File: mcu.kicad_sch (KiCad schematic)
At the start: 1 part, among them U1 PIC32CK1025GC01100-I/4SB

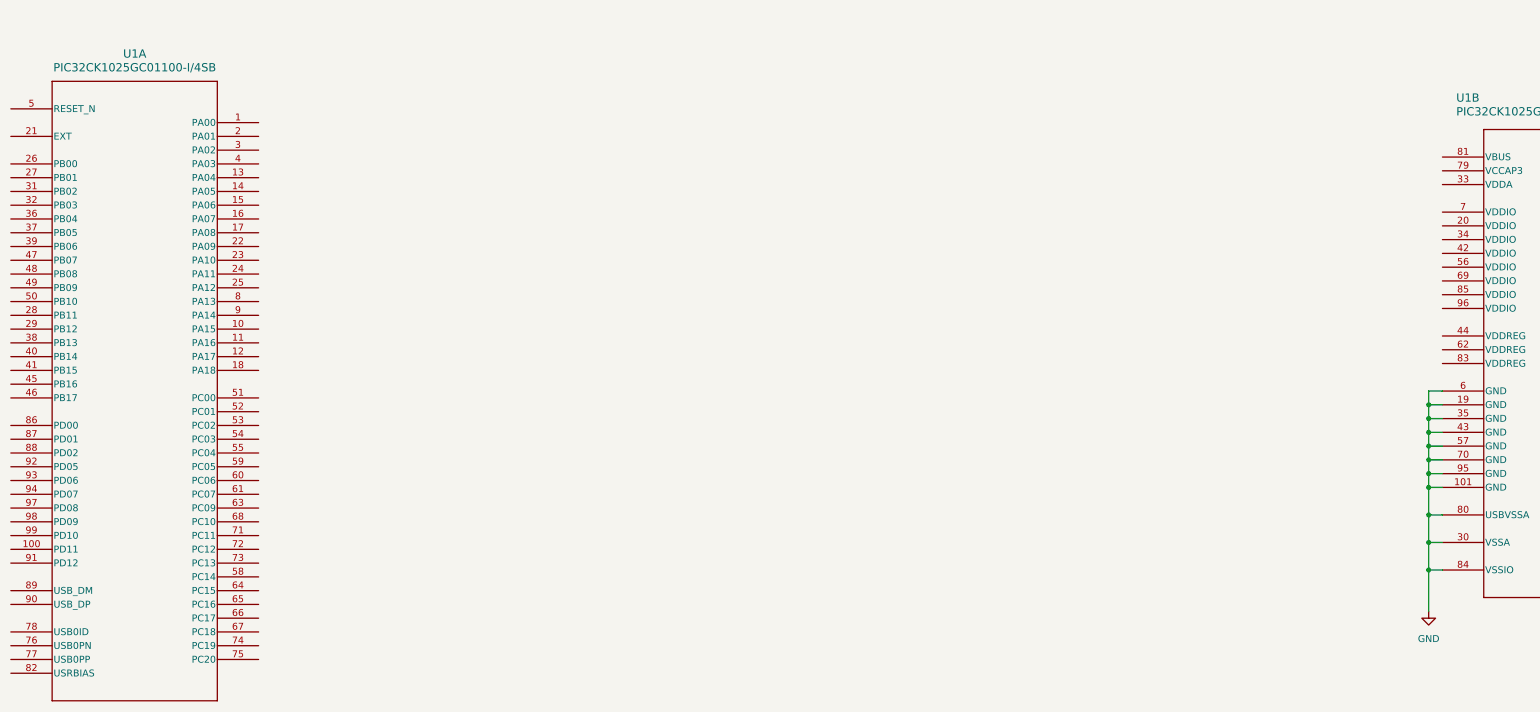
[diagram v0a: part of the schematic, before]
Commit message: did stuff
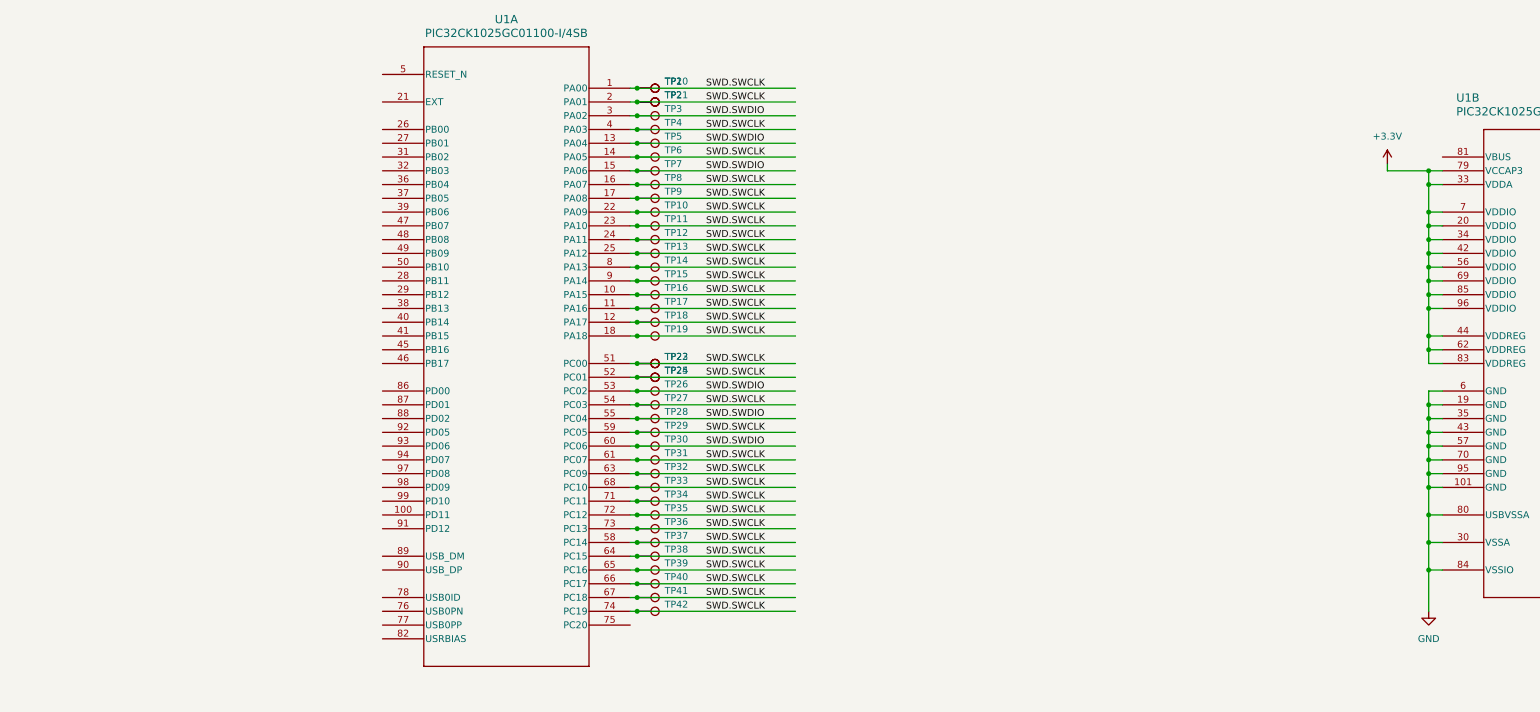
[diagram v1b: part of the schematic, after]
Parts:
- added TP1, TP10, TP11, TP12, TP13, TP14, TP15, TP16, TP17, TP18, TP19, TP2, TP20, TP21, TP22, TP23, TP24, TP25, TP26, TP27, TP28, TP29, TP3, TP30, TP31, TP32, TP33, TP34, TP35, TP36, TP37, TP38, TP39, TP4, TP40, TP41, TP42, TP5, TP6, TP7, TP8, TP9: TestPoint, symbol Connector:TestPoint
- U1: footprint TQFP100_4SB_6p3EP_MCH -> PIC32CK1025GC01100-I-4SB:TQFP100_4SB_6p3EP_MCH
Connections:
- net +3.3V: now reaches U1.20 (VDDIO)
- net +3.3V: now also U1.33 (VDDA), U1.34 (VDDIO), U1.42 (VDDIO), U1.44 (VDDREG), U1.56 (VDDIO), U1.62 (VDDREG), U1.69 (VDDIO), U1.7 (VDDIO), U1.79 (VCCAP3), U1.83 (VDDREG), U1.85 (VDDIO), U1.96 (VDDIO)
- net SWD.SWCLK: now reaches U1.1 (PA00)
- net SWD.SWCLK: now also U1.10 (PA15), U1.11 (PA16), U1.12 (PA17), U1.14 (PA05), U1.16 (PA07), U1.17 (PA08), U1.18 (PA18), U1.2 (PA01), U1.22 (PA09), U1.23 (PA10), U1.24 (PA11), U1.25 (PA12), U1.4 (PA03), U1.51 (PC00), U1.52 (PC01), U1.54 (PC03), U1.58 (PC14), U1.59 (PC05), U1.61 (PC07), U1.63 (PC09), U1.64 (PC15), U1.65 (PC16), U1.66 (PC17), U1.67 (PC18), U1.68 (PC10), U1.71 (PC11), U1.72 (PC12), U1.73 (PC13), U1.74 (PC19), U1.8 (PA13), U1.9 (PA14), TP1.1, TP10.1, TP11.1, TP12.1, TP13.1, TP14.1, TP15.1, TP16.1, TP17.1, TP18.1, TP19.1, TP2.1, TP20.1, TP21.1, TP22.1, TP23.1, TP24.1, TP25.1, TP27.1, TP29.1, TP31.1, TP32.1, TP33.1, TP34.1, TP35.1, TP36.1, TP37.1, TP38.1, TP39.1, TP4.1, TP40.1, TP41.1, TP42.1, TP6.1, TP8.1, TP9.1
- net SWD.SWDIO: now reaches U1.13 (PA04)
- net SWD.SWDIO: now also U1.15 (PA06), U1.3 (PA02), U1.53 (PC02), U1.55 (PC04), U1.60 (PC06), TP26.1, TP28.1, TP3.1, TP30.1, TP5.1, TP7.1
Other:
- moved on the sheet: U1A

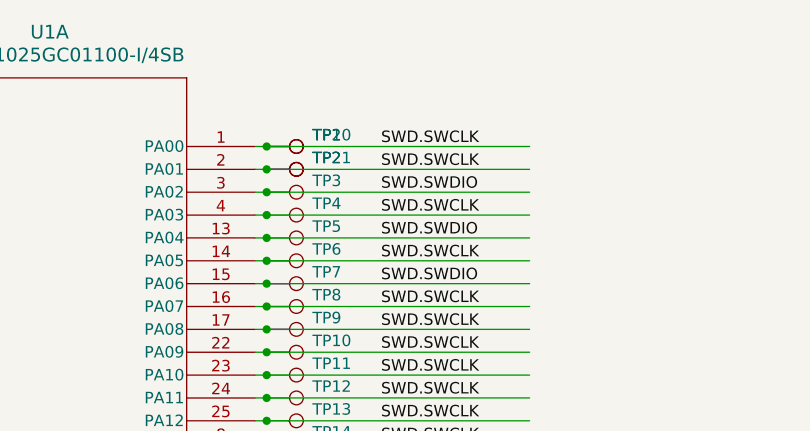
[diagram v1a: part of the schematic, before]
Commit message: stuff
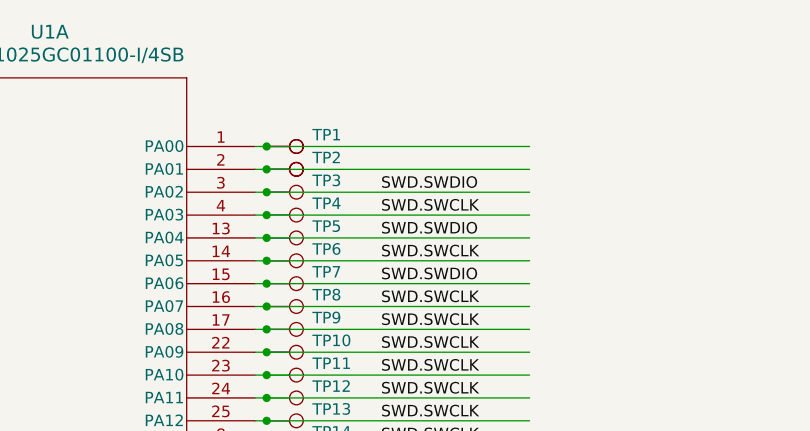
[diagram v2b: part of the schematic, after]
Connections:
- net SWD.SWCLK: no longer TP1.1, TP2.1, TP20.1, TP21.1, U1.1 (PA00), U1.2 (PA01)
- new net: TP2.1, TP21.1, U1.2 (PA01)
- new net: TP1.1, TP20.1, U1.1 (PA00)
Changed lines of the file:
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@@
-		)
-	)
-	(label "SWD.SWCLK"
-		(at 196.85 76.2 0)
-		(effects
-			(font
-				(size 1.27 1.27)
-			)
-			(justify left bottom)
-		)
-	)
-	(label "SWD.SWCLK"
-		(at 196.85 78.74 0)
-		(effects
-			(font
-				(size 1.27 1.27)
-			)
-			(justify left bottom)
 		)
 	)
@@
 				)
 				(justify left)
+				(hide yes)
 			)
 		)
@@
 				)
 				(justify left)
-			)
-		)
+				(hide yes)
+			)
+		)

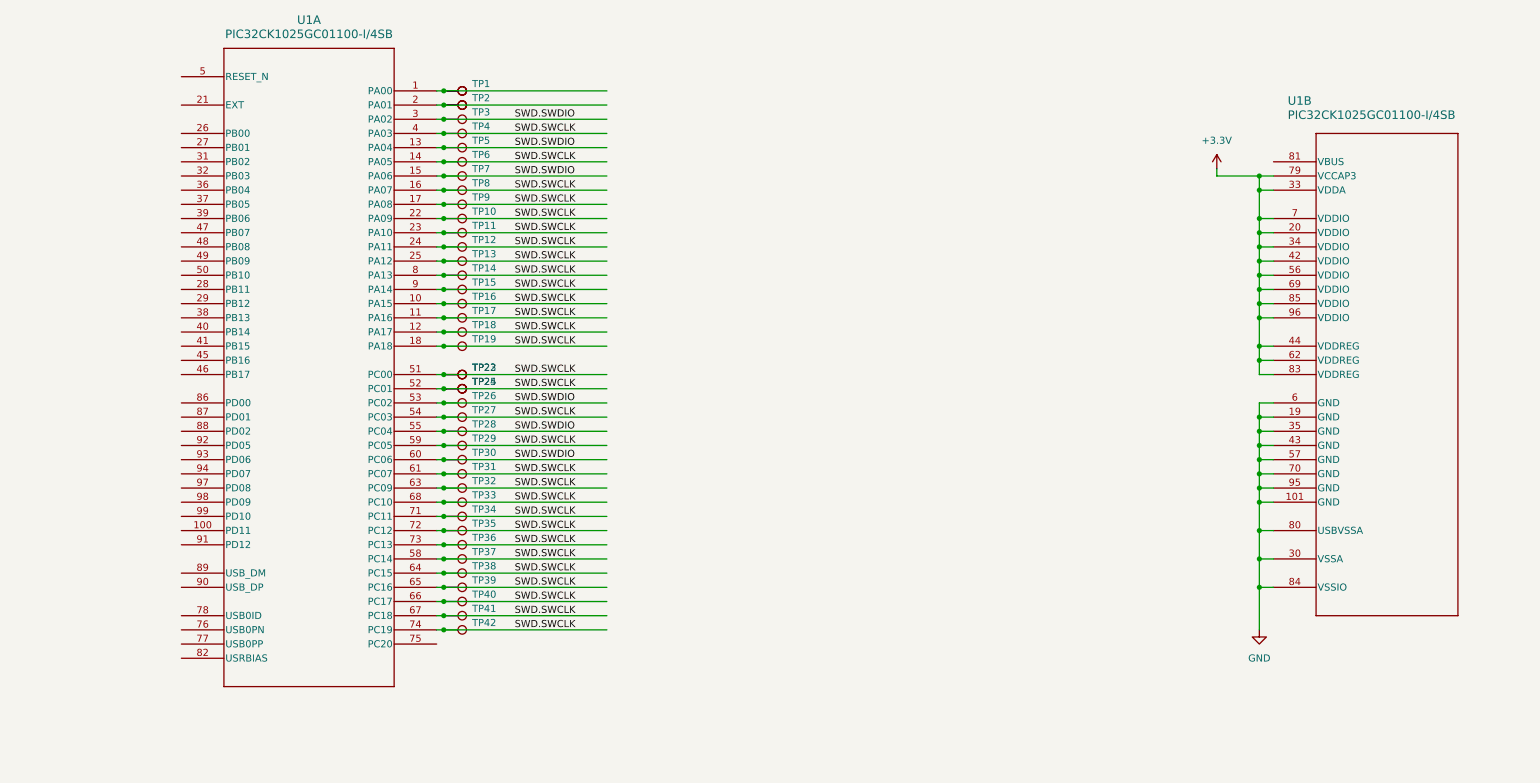
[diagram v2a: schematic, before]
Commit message: stuff
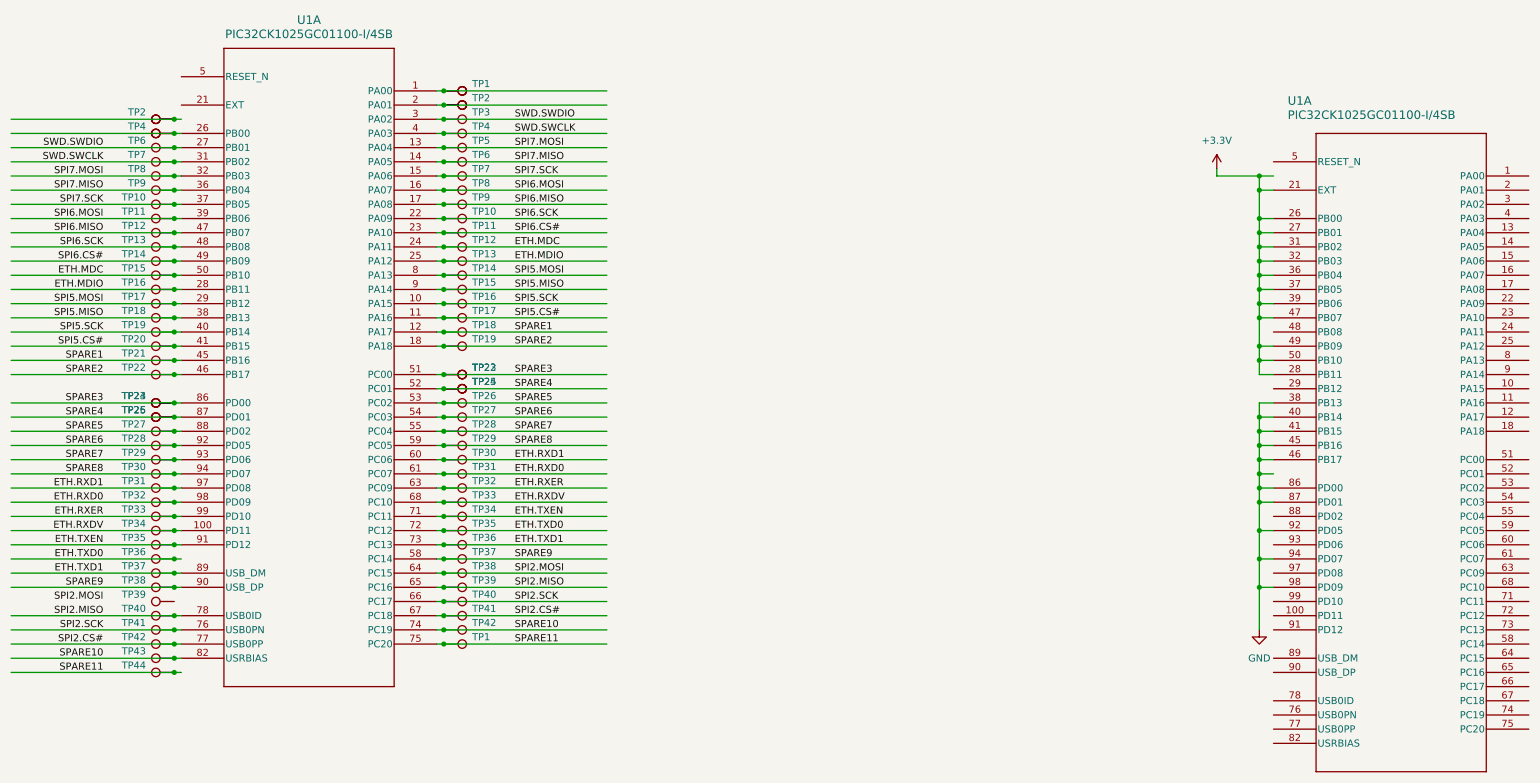
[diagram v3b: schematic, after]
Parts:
- added TP1, TP10, TP11, TP12, TP13, TP14, TP15, TP16, TP17, TP18, TP19, TP2, TP20, TP21, TP22, TP23, TP24, TP25, TP26, TP27, TP28, TP29, TP3, TP30, TP31, TP32, TP33, TP34, TP35, TP36, TP37, TP38, TP39, TP4, TP40, TP41, TP42, TP43, TP44, TP5, TP6, TP7, TP8, TP9: TestPoint, symbol Connector:TestPoint
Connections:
- net +3.3V: now also U1.21 (EXT), U1.26 (PB00), U1.27 (PB01), U1.28 (PB11), U1.31 (PB02), U1.32 (PB03), U1.36 (PB04), U1.37 (PB05), U1.39 (PB06), U1.47 (PB07), U1.49 (PB09), U1.50 (PB10); no longer U1.20 (VDDIO), U1.33 (VDDA), U1.34 (VDDIO), U1.42 (VDDIO), U1.44 (VDDREG), U1.56 (VDDIO), U1.62 (VDDREG), U1.69 (VDDIO), U1.7 (VDDIO), U1.79 (VCCAP3), U1.83 (VDDREG), U1.85 (VDDIO), U1.96 (VDDIO)
- net GND: now also U1.38 (PB13), U1.40 (PB14), U1.41 (PB15), U1.45 (PB16), U1.46 (PB17), U1.86 (PD00), U1.87 (PD01), U1.92 (PD05), U1.94 (PD07), U1.98 (PD09); no longer U1.101 (GND), U1.19 (GND), U1.30 (VSSA), U1.35 (GND), U1.43 (GND), U1.57 (GND), U1.6 (GND), U1.70 (GND), U1.80 (USBVSSA), U1.84 (VSSIO), U1.95 (GND)
- net SWD.SWCLK: now also U1.31 (PB02), TP7.1; no longer TP10.1, TP11.1, TP12.1, TP13.1, TP14.1, TP15.1, TP16.1, TP17.1, TP18.1, TP19.1, TP22.1, TP23.1, TP24.1, TP25.1, TP27.1, TP29.1, TP31.1, TP32.1, TP33.1, TP34.1, TP35.1, TP36.1, TP37.1, TP38.1, TP39.1, TP40.1, TP41.1, TP42.1, TP6.1, TP8.1, TP9.1, U1.10 (PA15), U1.11 (PA16), U1.12 (PA17), U1.14 (PA05), U1.16 (PA07), U1.17 (PA08), U1.18 (PA18), U1.22 (PA09), U1.23 (PA10), U1.24 (PA11), U1.25 (PA12), U1.51 (PC00), U1.52 (PC01), U1.54 (PC03), U1.58 (PC14), U1.59 (PC05), U1.61 (PC07), U1.63 (PC09), U1.64 (PC15), U1.65 (PC16), U1.66 (PC17), U1.67 (PC18), U1.68 (PC10), U1.71 (PC11), U1.72 (PC12), U1.73 (PC13), U1.74 (PC19), U1.8 (PA13), U1.9 (PA14)
- net SWD.SWDIO: now also U1.27 (PB01), TP6.1; no longer TP26.1, TP28.1, TP30.1, TP5.1, TP7.1, U1.13 (PA04), U1.15 (PA06), U1.53 (PC02), U1.55 (PC04), U1.60 (PC06)
- net ETH.RXDV: now reaches U1.100 (PD11)
- net ETH.RXDV: now also TP33.1, U1.68 (PC10), TP34.1
- net at U1.26 (PB00): now also TP4.1, TP5.1
- net ETH.MDIO: now reaches U1.28 (PB11)
- net ETH.MDIO: now also TP13.1, U1.25 (PA12), TP16.1
- net SPI5.MOSI: now reaches U1.29 (PB12)
- net SPI5.MOSI: now also TP14.1, U1.8 (PA13), TP17.1
- net SPI7.MOSI: now reaches U1.32 (PB03)
- net SPI7.MOSI: now also TP5.1, U1.13 (PA04), TP8.1
- net SPI7.MISO: now reaches U1.36 (PB04)
- net SPI7.MISO: now also TP6.1, U1.14 (PA05), TP9.1
- net SPI7.SCK: now reaches U1.37 (PB05)
- net SPI7.SCK: now also TP7.1, U1.15 (PA06), TP10.1
- net SPI5.MISO: now reaches U1.38 (PB13)
- net SPI5.MISO: now also TP15.1, U1.9 (PA14), TP18.1
- net SPI6.MOSI: now reaches U1.39 (PB06)
- net SPI6.MOSI: now also TP8.1, U1.16 (PA07), TP11.1
- net SPI5.SCK: now reaches U1.40 (PB14)
- net SPI5.SCK: now also TP16.1, U1.10 (PA15), TP19.1
- net SPI5.CS#: now reaches U1.41 (PB15)
- net SPI5.CS#: now also TP17.1, U1.11 (PA16), TP20.1
- net SPARE1: now reaches U1.45 (PB16)
- net SPARE1: now also TP18.1, U1.12 (PA17), TP21.1
- net SPARE2: now reaches U1.46 (PB17)
- net SPARE2: now also TP19.1, U1.18 (PA18), TP22.1
- net SPI6.MISO: now reaches U1.47 (PB07)
- net SPI6.MISO: now also TP9.1, U1.17 (PA08), TP12.1
- net SPI6.SCK: now reaches U1.48 (PB08)
- net SPI6.SCK: now also TP10.1, U1.22 (PA09), TP13.1
- net SPI6.CS#: now reaches U1.49 (PB09)
- net SPI6.CS#: now also TP11.1, U1.23 (PA10), TP14.1
- net ETH.MDC: now reaches U1.50 (PB10)
- net ETH.MDC: now also TP12.1, U1.24 (PA11), TP15.1
- net SPARE11: now reaches U1.75 (PC20)
- net SPARE11: now also TP1.1, TP44.1
- net SPI2.SCK: now reaches U1.76 (USB0PN)
- net SPI2.SCK: now also TP40.1, U1.66 (PC17), TP41.1
- net SPI2.CS#: now reaches U1.77 (USB0PP)
- net SPI2.CS#: now also TP41.1, U1.67 (PC18), TP42.1
- net SPI2.MISO: now reaches U1.78 (USB0ID)
- net SPI2.MISO: now also TP39.1, U1.65 (PC16), TP40.1
- net SPARE10: now reaches U1.82 (USRBIAS)
- net SPARE10: now also TP42.1, U1.74 (PC19), TP43.1
- net SPARE3: now reaches U1.86 (PD00)
- net SPARE3: now also TP22.1, TP23.1, U1.51 (PC00), TP23.1, TP24.1
- net SPARE4: now reaches U1.87 (PD01)
- net SPARE4: now also TP24.1, TP25.1, U1.52 (PC01), TP25.1, TP26.1
- net SPARE5: now reaches U1.88 (PD02)
- net SPARE5: now also TP26.1, U1.53 (PC02), TP27.1
- net ETH.TXD1: now reaches U1.89 (USB_DM)
- net ETH.TXD1: now also TP36.1, U1.73 (PC13), TP37.1
- net SPARE9: now reaches U1.90 (USB_DP)
- net SPARE9: now also TP37.1, U1.58 (PC14), TP38.1
- net ETH.TXEN: now reaches U1.91 (PD12)
- net ETH.TXEN: now also TP34.1, U1.71 (PC11), TP35.1
- net SPARE6: now reaches U1.92 (PD05)
- net SPARE6: now also TP27.1, U1.54 (PC03), TP28.1
- net SPARE7: now reaches U1.93 (PD06)
- net SPARE7: now also TP28.1, U1.55 (PC04), TP29.1
- net SPARE8: now reaches U1.94 (PD07)
- net SPARE8: now also TP29.1, U1.59 (PC05), TP30.1
- net ETH.RXD1: now reaches U1.97 (PD08)
- net ETH.RXD1: now also TP30.1, U1.60 (PC06), TP31.1
- net ETH.RXD0: now reaches U1.98 (PD09)
- net ETH.RXD0: now also TP31.1, U1.61 (PC07), TP32.1
- net ETH.RXER: now reaches U1.99 (PD10)
- net ETH.RXER: now also TP32.1, U1.63 (PC09), TP33.1
- new net: TP2.1, TP3.1
- new net ETH.TXD0: TP35.1, TP36.1, U1.72 (PC12)
- new net SPI2.MOSI: TP38.1, U1.64 (PC15)
